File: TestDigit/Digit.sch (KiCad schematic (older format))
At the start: 2 parts

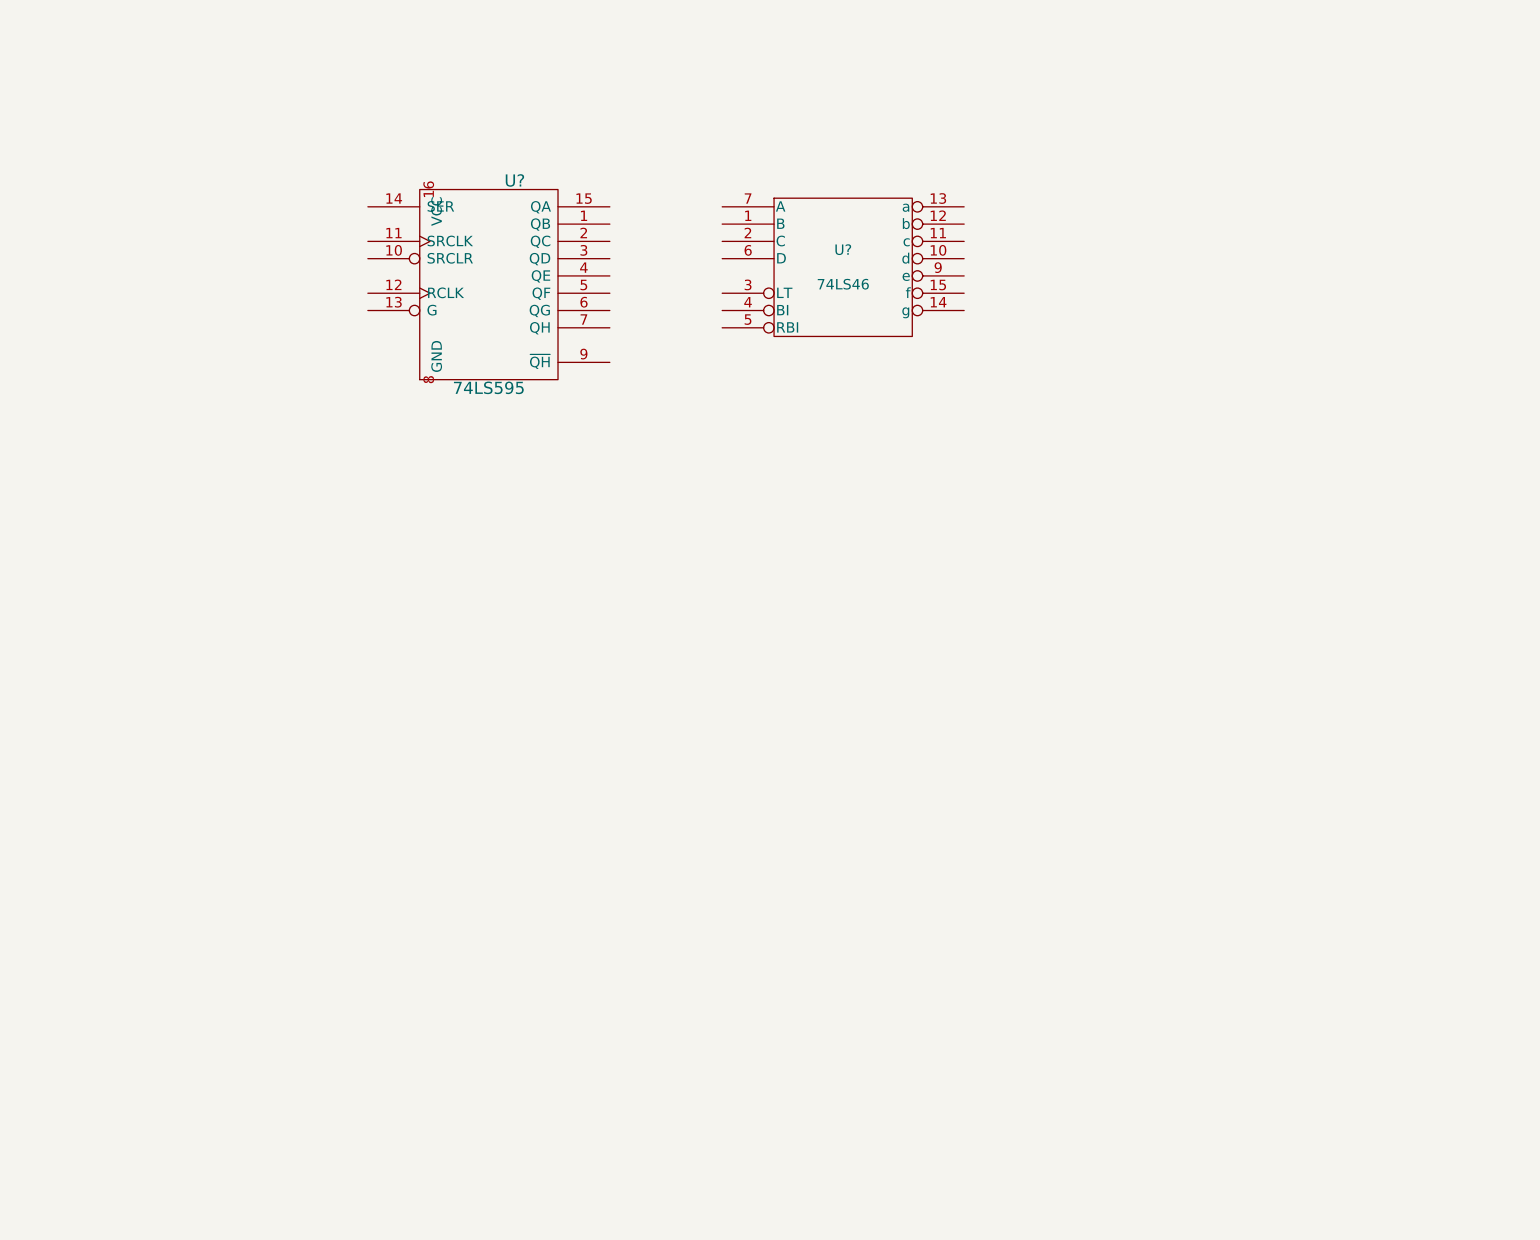
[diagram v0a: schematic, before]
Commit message: Digit PCB
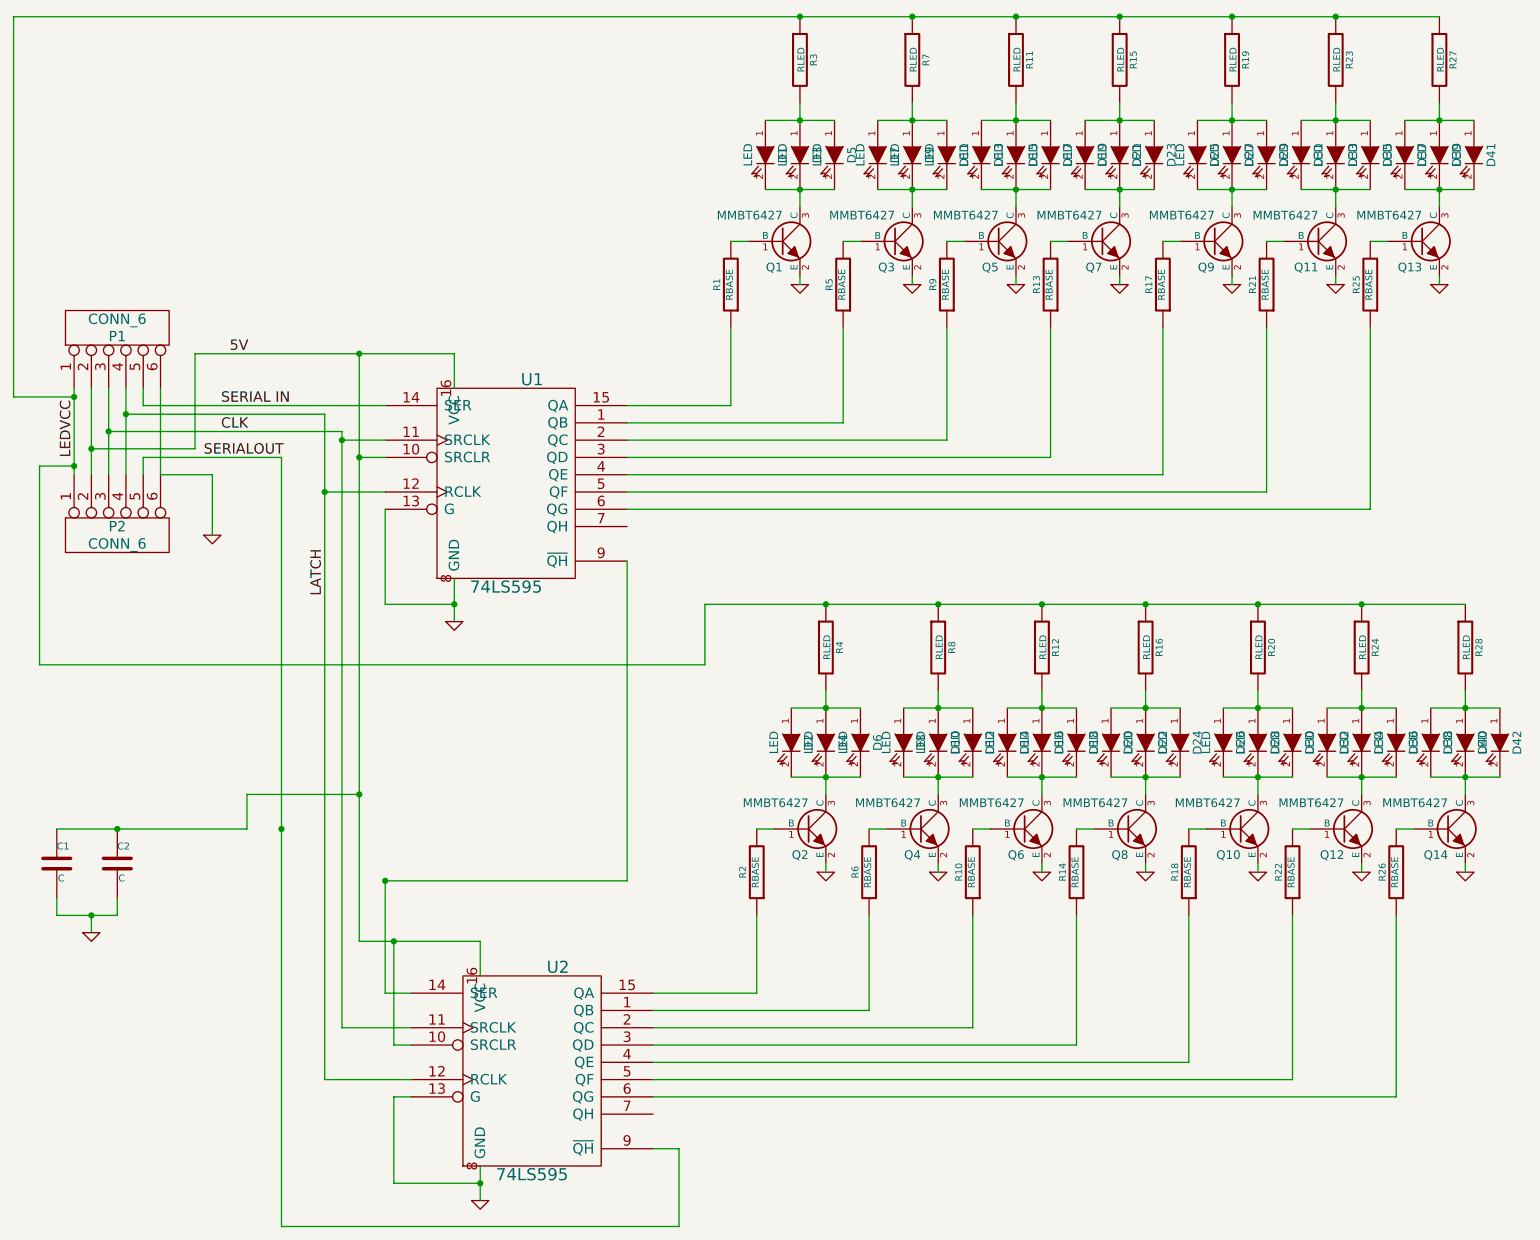
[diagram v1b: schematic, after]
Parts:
- removed U?: 74LS46, ~, symbol 74LS46
- added C1, C2: C, ~, symbol C
- added D1, D10, D11, D12, D13, D14, D15, D16, D17, D18, D19, D2, D20, D21, D22, D23, D24, D25, D26, D27, D28, D29, D3, D30, D31, D32, D33, D34, D35, D36, D37, D38, D39, D4, D40, D41, D42, D5, D6, D7, D8, D9: LED, ~, symbol LED
- added P1, P2: CONN_6, symbol CONN_6
- added Q1, Q10, Q11, Q12, Q13, Q14, Q2, Q3, Q4, Q5, Q6, Q7, Q8, Q9: MMBT6427, ~, symbol MMBT6427
- added R1, R10, R13, R14, R17, R18, R2, R21, R22, R25, R26, R5, R6, R9: RBASE, ~, symbol R
- added R11, R12, R15, R16, R19, R20, R23, R24, R27, R28, R3, R4, R7, R8: RLED, ~, symbol R
- added U2: 74LS595, ~, symbol 74LS595
- gave numbers to parts that had none: 1
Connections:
- net GND: now also U1.13 (G), U1.8 (GND), C1.2, C2.2, P1.6, P2.6, Q1.2 (E), Q10.2 (E), Q11.2 (E), Q12.2 (E), Q13.2 (E), Q14.2 (E), Q2.2 (E), Q3.2 (E), Q4.2 (E), Q5.2 (E), Q6.2 (E), Q7.2 (E), Q8.2 (E), Q9.2 (E), U2.13 (G), U2.8 (GND)
- net at U1.1 (QB): now also R5.1
- net 5V: now reaches U1.10 (SRCLR)
- net 5V: now also U1.16 (VCC), C1.1, C2.1, P1.2, P2.2, U2.10 (SRCLR), U2.16 (VCC)
- net CLK: now reaches U1.11 (SRCLK)
- net CLK: now also P1.3, P2.3, U2.11 (SRCLK)
- net LATCH: now reaches U1.12 (RCLK)
- net LATCH: now also P1.4, P2.4, U2.12 (RCLK)
- net SERIAL IN: now reaches U1.14 (SER)
- net SERIAL IN: now also P1.5
- net at U1.15 (QA): now also R1.1
- net at U1.2 (QC): now also R9.1
- net at U1.3 (QD): now also R13.1
- net at U1.4 (QE): now also R17.1
- net at U1.5 (QF): now also R21.1
- net at U1.6 (QG): now also R25.1
- net at U1.9 (~QH): now also U2.14 (SER)
- new net: Q1.1 (B), R1.2
- new net: D1.2 (K), D3.2 (K), D5.2 (K), Q1.3 (C)
- new net: Q3.1 (B), R5.2
- new net: D11.2 (K), D7.2 (K), D9.2 (K), Q3.3 (C)
- new net: Q5.1 (B), R9.2
- new net: D13.2 (K), D15.2 (K), D17.2 (K), Q5.3 (C)
- new net: Q7.1 (B), R13.2
- new net: D19.2 (K), D21.2 (K), D23.2 (K), Q7.3 (C)
- new net: Q9.1 (B), R17.2
- new net: D25.2 (K), D27.2 (K), D29.2 (K), Q9.3 (C)
- new net: Q11.1 (B), R21.2
- new net: D31.2 (K), D33.2 (K), D35.2 (K), Q11.3 (C)
- new net: Q13.1 (B), R25.2
- new net: D37.2 (K), D39.2 (K), D41.2 (K), Q13.3 (C)
- new net: D1.1 (A), D3.1 (A), D5.1 (A), R3.2
- new net: D11.1 (A), D7.1 (A), D9.1 (A), R7.2
- new net: D13.1 (A), D15.1 (A), D17.1 (A), R11.2
- new net: D19.1 (A), D21.1 (A), D23.1 (A), R15.2
- new net: D25.1 (A), D27.1 (A), D29.1 (A), R19.2
- new net: D31.1 (A), D33.1 (A), D35.1 (A), R23.2
- new net: D37.1 (A), D39.1 (A), D41.1 (A), R27.2
- new net: R6.1, U2.1 (QB)
- new net: R2.1, U2.15 (QA)
- new net: R10.1, U2.2 (QC)
- new net: R14.1, U2.3 (QD)
- new net: R18.1, U2.4 (QE)
- new net: R22.1, U2.5 (QF)
- new net: R26.1, U2.6 (QG)
- new net: Q2.1 (B), R2.2
- new net: D2.2 (K), D4.2 (K), D6.2 (K), Q2.3 (C)
- new net: Q4.1 (B), R6.2
- new net: D10.2 (K), D12.2 (K), D8.2 (K), Q4.3 (C)
- new net: Q6.1 (B), R10.2
- new net: D14.2 (K), D16.2 (K), D18.2 (K), Q6.3 (C)
- new net: Q8.1 (B), R14.2
- new net: D20.2 (K), D22.2 (K), D24.2 (K), Q8.3 (C)
- new net: Q10.1 (B), R18.2
- new net: D26.2 (K), D28.2 (K), D30.2 (K), Q10.3 (C)
- new net: Q12.1 (B), R22.2
- new net: D32.2 (K), D34.2 (K), D36.2 (K), Q12.3 (C)
- new net: Q14.1 (B), R26.2
- new net: D38.2 (K), D40.2 (K), D42.2 (K), Q14.3 (C)
- new net: D2.1 (A), D4.1 (A), D6.1 (A), R4.2
- new net: D10.1 (A), D12.1 (A), D8.1 (A), R8.2
- new net: D14.1 (A), D16.1 (A), D18.1 (A), R12.2
- new net: D20.1 (A), D22.1 (A), D24.1 (A), R16.2
- new net: D26.1 (A), D28.1 (A), D30.1 (A), R20.2
- new net: D32.1 (A), D34.1 (A), D36.1 (A), R24.2
- new net: D38.1 (A), D40.1 (A), D42.1 (A), R28.2
- new net LEDVCC: P1.1, P2.1, R11.1, R12.1, R15.1, R16.1, R19.1, R20.1, R23.1, R24.1, R27.1, R28.1, R3.1, R4.1, R7.1, R8.1
- new net SERIALOUT: P2.5, U2.9 (~QH)
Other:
- moved on the sheet: U1
